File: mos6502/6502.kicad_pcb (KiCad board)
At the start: 2 copper layers, 4 parts, among them U2 74HC245, U3 74HC245, U4 74HC245, U5 WD65C02

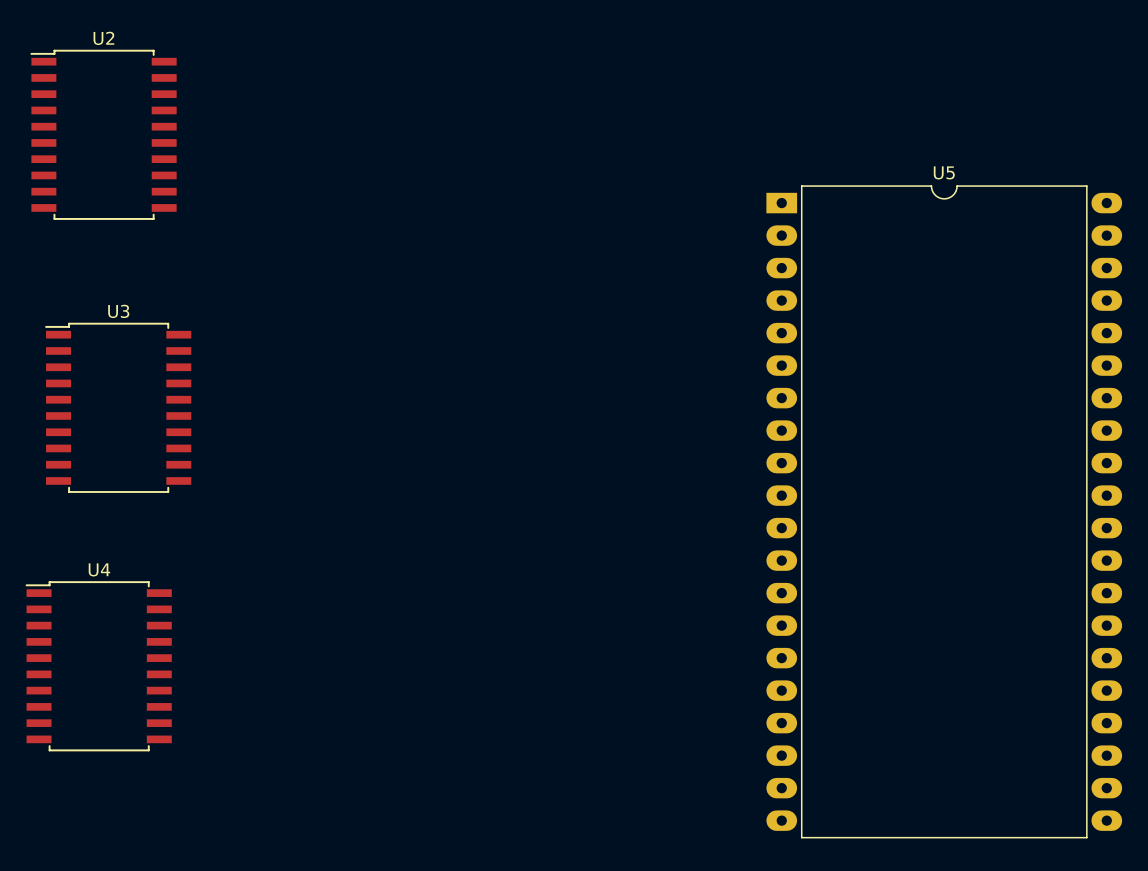
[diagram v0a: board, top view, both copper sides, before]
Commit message: update for PCB order
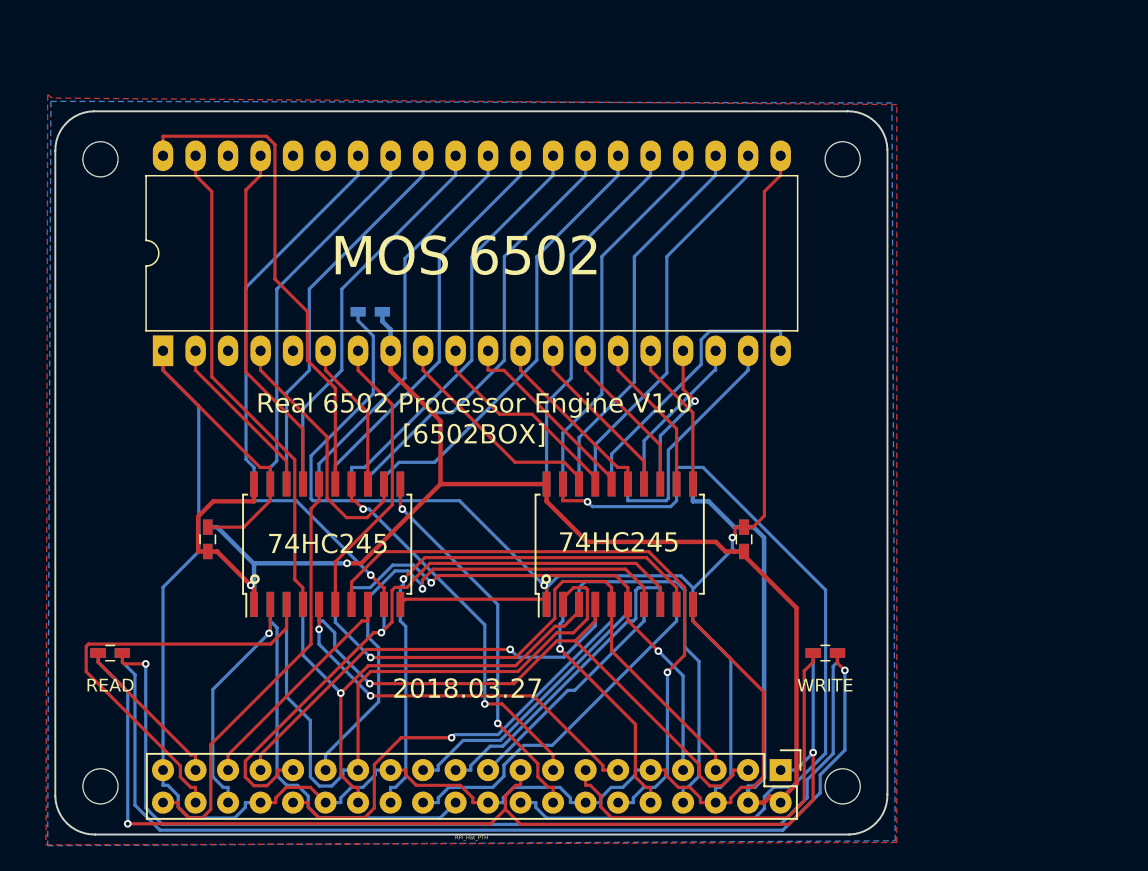
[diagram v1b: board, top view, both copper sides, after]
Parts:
- added C1: C, Capacitors_SMD:C_0603_HandSoldering, F.Cu at (146.1, 95.2)
- added C2: C, Capacitors_SMD:C_0603_HandSoldering, F.Cu at (188.0, 95.2)
- added C3: C, Capacitors_SMD:C_0603_HandSoldering, B.Cu at (146.1, 95.2)
- added C4: C, Capacitors_SMD:C_0603_HandSoldering, B.Cu at (188.0, 95.2)
- added C5: C, Capacitors_SMD:C_0603_HandSoldering, B.Cu at (158.8, 77.5)
- added D1: LED, Capacitors_SMD:C_0603_HandSoldering, F.Cu at (138.4, 104.1)
- added D2: LED, Capacitors_SMD:C_0603_HandSoldering, F.Cu at (194.3, 104.1)
- added J1: Raspberry_Pi_2_3, Pin_Headers:Pin_Header_Straight_2x20, F.Cu at (190.8, 113.3)
- added R1: R, Capacitors_SMD:C_0603_HandSoldering, B.Cu at (194.3, 104.1)
- added R2: R, Capacitors_SMD:C_0603_HandSoldering, B.Cu at (138.4, 104.1)
- added REF**: RPi_Hat_PTH, msx:z_RPi_Hat_layout, F.Cu at (166.7, 90.1)
- added U1: 74HC245, Housings_SOIC:SOIC-20W_7.5x12.8mm_Pitch1.27mm, B.Cu at (178.2, 95.6)
- U3: moved to B.Cu
- U5: footprint Housings_DIP:DIP-40_W25.4mm_LongPads -> Housings_DIP:DIP-40_W15.24mm_LongPads
- moved U5 49.7 mm to (142.6, 80.5), turned to 90 degrees
- moved U4 41.8 mm to (178.2, 95.6), turned to 90 degrees
- moved U2 36.4 mm to (155.4, 95.6), turned to 90 degrees
- moved U3 19.5 mm to (155.4, 95.6), turned to 270 degrees
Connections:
- U2 pad 1: GND -> VCC
- U5 pad 4: /NC -> /IRQ
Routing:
- net GND: track 0.00 -> 256.5 mm, vias 0 -> 2
- net VCC: track 0.00 -> 137.7 mm, vias 0 -> 2
- net /3V3: track 0.00 -> 88.0 mm, vias 0 -> 2
- net Net-(D2-Pad2): track 0.00 -> 79.8 mm, vias 0 -> 1
- net Net-(D1-Pad2): track 0.00 -> 79.2 mm, vias 0 -> 1
- net /RC24: track 0.00 -> 68.7 mm, vias 0 -> 1
- net /RD0: track 0.00 -> 50.9 mm
- net /RD6: track 0.00 -> 50.7 mm, vias 0 -> 1
- net /RC18: track 0.00 -> 50.1 mm, vias 0 -> 1
- net /RD2: track 0.00 -> 48.4 mm, vias 0 -> 1
- net /RD3: track 0.00 -> 45.7 mm, vias 0 -> 1
- net /RW: track 0.00 -> 45.1 mm, vias 0 -> 1
- net /RD7: track 0.00 -> 42.8 mm, vias 0 -> 1
- net /RD5: track 0.00 -> 41.7 mm, vias 0 -> 1
- net /RD4: track 0.00 -> 40.9 mm, vias 0 -> 2
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- added copper zone on B.Cu, net GND
- added copper zone on F.Cu, net GND
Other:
- board outline added: 65 x 56.5 mm
- net class VCC added: clearance 0.2, trace_width 0.35, via_dia 0.6, via_drill 0.4
- board text added: "2018.03.27"
- board text added: "74HC245"
- board text added: "MOS 6502"
- board text added: "READ"
- board text added: "Real 6502 Processor Engine V1.0 [6502BOX]"
- board text added: "WRITE"
- board text added: "meeso.kim@gmail.com 2018.03.27"
